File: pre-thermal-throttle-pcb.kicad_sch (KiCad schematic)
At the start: 70 parts, among them IC1 LMR51420XFDDCR, IC2 ADR02BRZ-REEL7, IC3 ADR02BRZ-REEL7, IC4 ADR02BRZ-REEL7, IC5 ADR02BRZ-REEL7, J1 RJHSE-5381-ND, J2 STEERING, J3 Motor Throttle Connector, J4 RJHSE-5381-ND, U1 SN65HVD230, U2 BMI088, U3 MAX3485CSA, U4 MCP3008, U5 ESP32-DevKitC

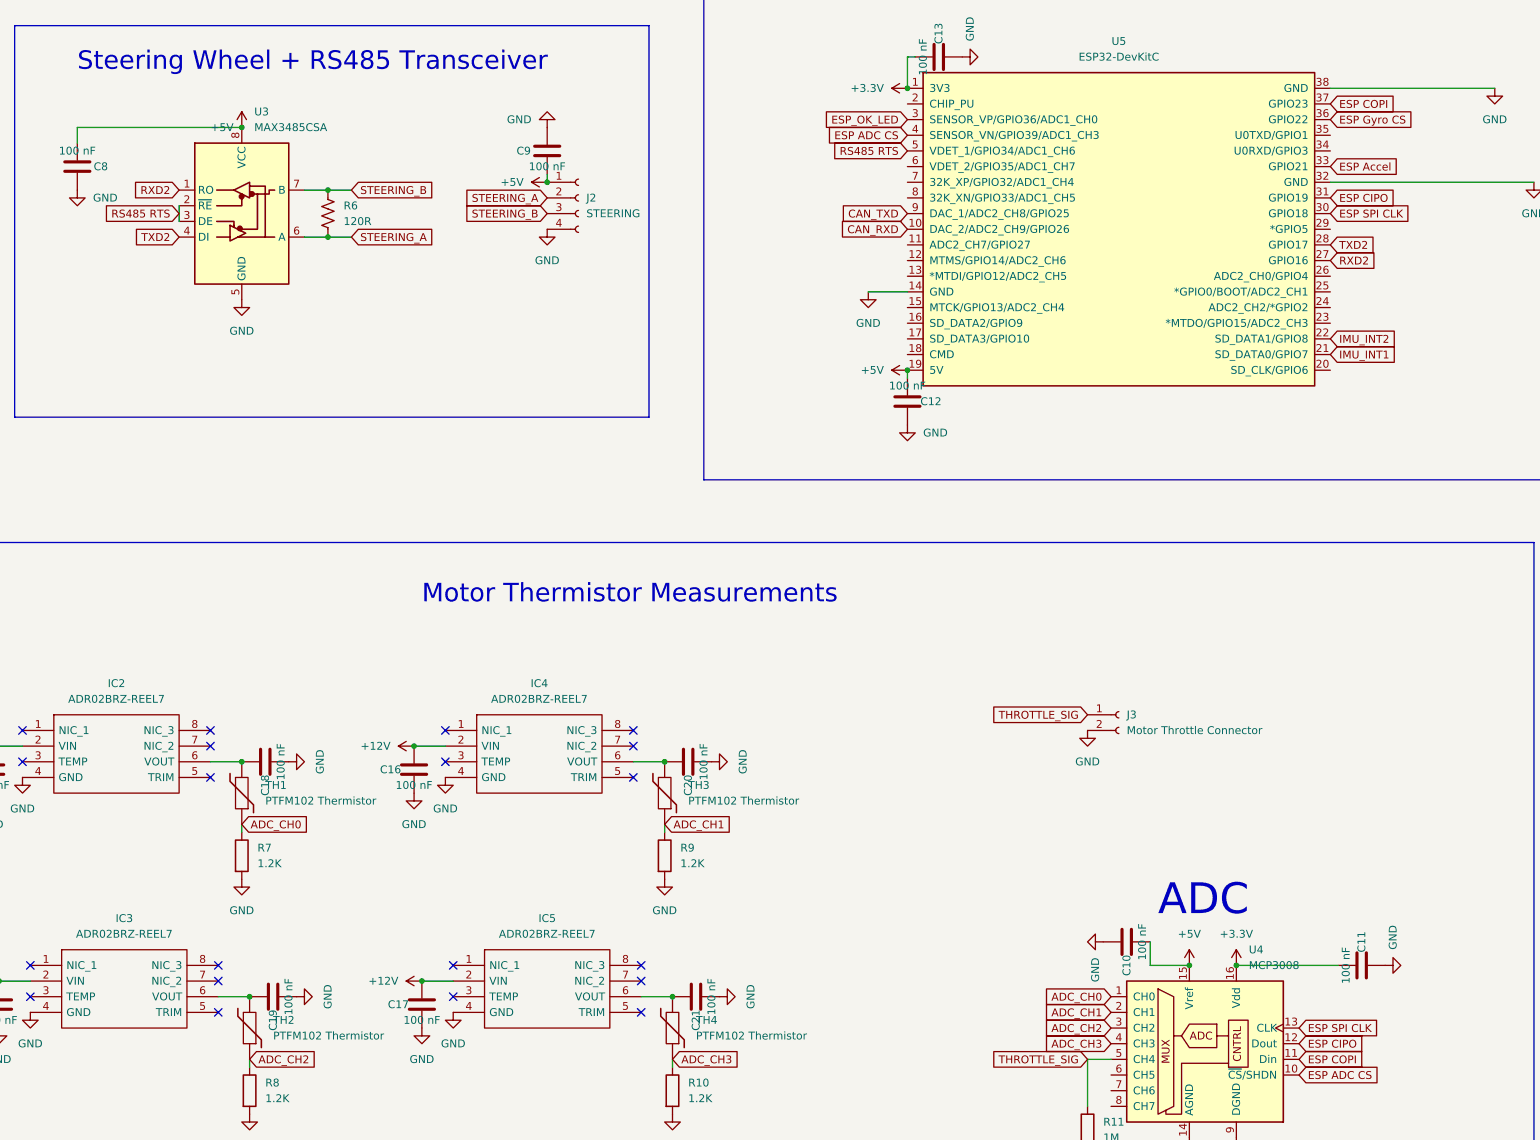
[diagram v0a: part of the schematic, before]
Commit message: Hopefully finished?
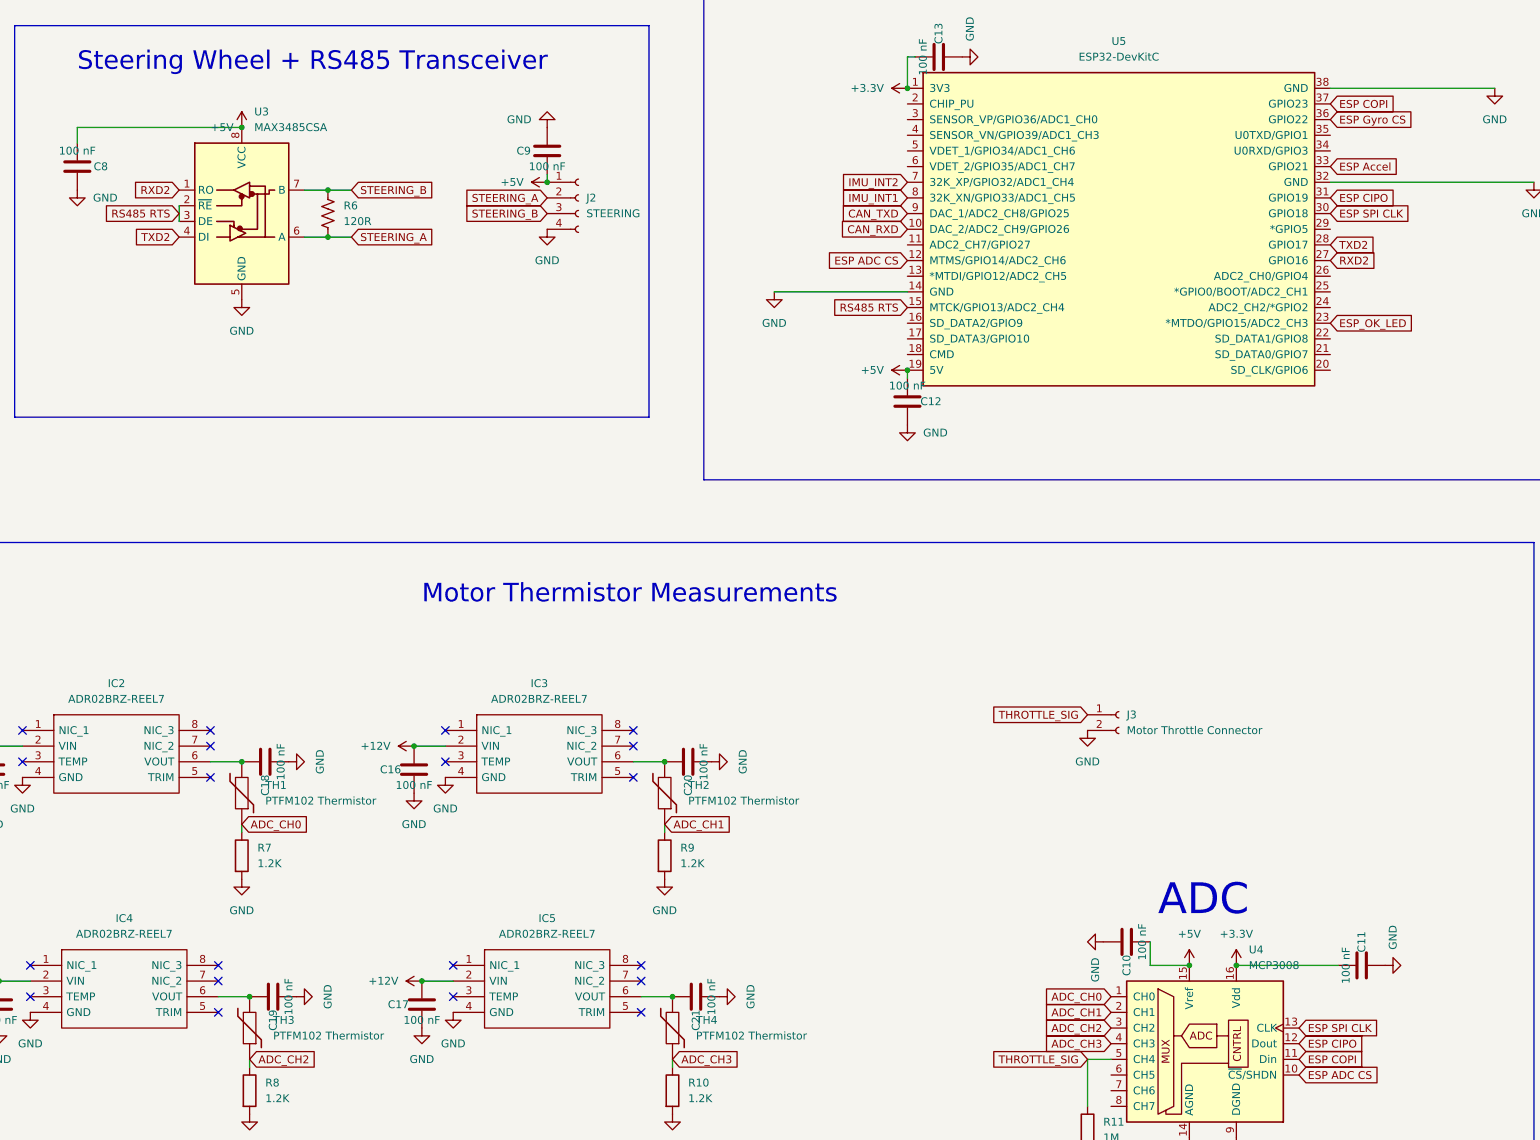
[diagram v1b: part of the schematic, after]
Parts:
- renumbered IC4 to IC3, IC3 to IC4, TH3 to TH2, TH2 to TH3
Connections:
- net ESP ADC CS: now also U5.12 (MTMS/GPIO14/ADC2_CH6); no longer U5.4 (SENSOR_VN/GPIO39/ADC1_CH3)
- net ESP_OK_LED: now also U5.23 (*MTDO/GPIO15/ADC2_CH3); no longer U5.3 (SENSOR_VP/GPIO36/ADC1_CH0)
- net IMU_INT1: now also U5.8 (32K_XN/GPIO33/ADC1_CH5); no longer U5.21 (SD_DATA0/GPIO7)
- net IMU_INT2: now also U5.7 (32K_XP/GPIO32/ADC1_CH4); no longer U5.22 (SD_DATA1/GPIO8)
- net RS485 RTS: now also U5.15 (MTCK/GPIO13/ADC2_CH4); no longer U5.5 (VDET_1/GPIO34/ADC1_CH6)
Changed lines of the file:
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@@
     (stroke (width 0) (type default) (color 0 0 0 0))
   )
-  (wire (pts (xy 302.26 233.68) (xy 308.61 233.68))
+  (wire (pts (xy 287.02 233.68) (xy 308.61 233.68))
     (stroke (width 0) (type default) (color 0 0 0 0))
   )
@@
     )
   )
+  (global_label "IMU_INT1" (shape input) (at 308.61 218.44 180) (fields_autoplaced)
+    (effects (font (size 1.27 1.27)) (justify right))
+    (property "Intersheet References" "${INTERSHEET_REFS}" (id 0) (at 297.7302 218.5194 0)
+      (effects (font (size 1.27 1.27)) (justify right) hide)
+    )
+  )
   (global_label "ESP SPI CLK" (shape input) (at 256.54 139.7 180) (fields_autoplaced)
     (effects (font (size 1.27 1.27)) (justify right))
@@
     )
   )
-  (global_label "IMU_INT2" (shape input) (at 377.19 241.3 0) (fields_autoplaced)
-    (effects (font (size 1.27 1.27)) (justify left))
-    (property "Intersheet References" "${INTERSHEET_REFS}" (id 0) (at 388.0698 241.2206 0)
-      (effects (font (size 1.27 1.27)) (justify left) hide)
-    )
-  )
   (global_label "STEERING_A" (shape input) (at 250.19 218.44 180) (fields_autoplaced)
     (effects (font (size 1.27 1.27)) (justify right))
@@
     )
   )
+  (global_label "RS485 RTS" (shape input) (at 308.61 236.22 180) (fields_autoplaced)
+    (effects (font (size 1.27 1.27)) (justify right))
+    (property "Intersheet References" "${INTERSHEET_REFS}" (id 0) (at 295.674 236.1406 0)
+      (effects (font (size 1.27 1.27)) (justify right) hide)
+    )
+  )
   (global_label "CAR_CANL" (shape input) (at 201.93 148.59 0) (fields_autoplaced)
     (effects (font (size 1.27 1.27)) (justify left))
@@
     )
   )
-  (global_label "IMU_INT1" (shape input) (at 377.19 243.84 0) (fields_autoplaced)
-    (effects (font (size 1.27 1.27)) (justify left))
-    (property "Intersheet References" "${INTERSHEET_REFS}" (id 0) (at 388.0698 243.7606 0)
-      (effects (font (size 1.27 1.27)) (justify left) hide)
-    )
-  )
   (global_label "CAN_TXD" (shape input) (at 167.64 143.51 180) (fields_autoplaced)
     (effects (font (size 1.27 1.27)) (justify right))
@@
     )
   )
+  (global_label "ESP_OK_LED" (shape input) (at 377.19 238.76 0) (fields_autoplaced)
+    (effects (font (size 1.27 1.27)) (justify left))
+    (property "Intersheet References" "${INTERSHEET_REFS}" (id 0) (at 391.2145 238.8394 0)
+      (effects (font (size 1.27 1.27)) (justify left) hide)
+    )
+  )
   (global_label "TXD2" (shape input) (at 190.5 224.79 180) (fields_autoplaced)
     (effects (font (size 1.27 1.27)) (justify right))
@@
     )
   )
-  (global_label "ESP Accel " (shape input) (at 256.54 132.08 180) (fields_autoplaced)
+  (global_label "IMU_INT2" (shape input) (at 308.61 215.9 180) (fields_autoplaced)
     (effects (font (size 1.27 1.27)) (justify right))
-    (property "Intersheet References" "${INTERSHEET_REFS}" (id 0) (at 243.5436 132.0006 0)
+    (property "Intersheet References" "${INTERSHEET_REFS}" (id 0) (at 297.7302 215.9794 0)
       (effects (font (size 1.27 1.27)) (justify right) hide)
     )
   )
-  (global_label "ADC_CH0" (shape input) (at 341.63 347.98 180) (fields_autoplaced)
+  (global_label "ESP Accel " (shape input) (at 256.54 132.08 180) (fields_autoplaced)
     (effects (font (size 1.27 1.27)) (justify right))
-    (property "Intersheet References" "${INTERSHEET_REFS}" (id 0) (at 330.8107 348.0594 0)
+    (property "Intersheet References" "${INTERSHEET_REFS}" (id 0) (at 243.5436 132.0006 0)
       (effects (font (size 1.27 1.27)) (justify right) hide)
     )
   )
-  (global_label "ESP ADC CS" (shape input) (at 308.61 208.28 180) (fields_autoplaced)
+  (global_label "ADC_CH0" (shape input) (at 341.63 347.98 180) (fields_autoplaced)
     (effects (font (size 1.27 1.27)) (justify right))
-    (property "Intersheet References" "${INTERSHEET_REFS}" (id 0) (at 294.525 208.3594 0)
+    (property "Intersheet References" "${INTERSHEET_REFS}" (id 0) (at 330.8107 348.0594 0)
       (effects (font (size 1.27 1.27)) (justify right) hide)
     )
@@
     )
   )
+  (global_label "ESP ADC CS" (shape input) (at 308.61 228.6 180) (fields_autoplaced)
+    (effects (font (size 1.27 1.27)) (justify right))
+    (property "Intersheet References" "${INTERSHEET_REFS}" (id 0) (at 294.525 228.6794 0)
+      (effects (font (size 1.27 1.27)) (justify right) hide)
+    )
+  )
   (global_label "ESP ADC CS" (shape input) (at 372.11 360.68 0) (fields_autoplaced)
     (effects (font (size 1.27 1.27)) (justify left))
@@
     )
   )
-  (global_label "RS485 RTS" (shape input) (at 308.61 210.82 180) (fields_autoplaced)
-    (effects (font (size 1.27 1.27)) (justify right))
-    (property "Intersheet References" "${INTERSHEET_REFS}" (id 0) (at 295.674 210.7406 0)
-      (effects (font (size 1.27 1.27)) (justify right) hide)
-    )
-  )
-  (global_label "ESP_OK_LED" (shape input) (at 308.61 205.74 180) (fields_autoplaced)
-    (effects (font (size 1.27 1.27)) (justify right))
-    (property "Intersheet References" "${INTERSHEET_REFS}" (id 0) (at 294.5855 205.6606 0)
-      (effects (font (size 1.27 1.27)) (justify right) hide)
-    )
-  )
   (global_label "ADC_CH1" (shape input) (at 269.24 320.04 0) (fields_autoplaced)
     (effects (font (size 1.27 1.27)) (justify left))
@@
   (symbol (lib_id "Device:Thermistor") (at 269.24 314.96 180) (unit 1)
     (in_bom yes) (on_board yes) (fields_autoplaced)
-    (property "Reference" "TH3" (id 0) (at 273.05 313.6899 0)
+    (property "Reference" "TH2" (id 0) (at 273.05 313.6899 0)
       (effects (font (size 1.27 1.27)) (justify right))
     )
@@
   (symbol (lib_id "Device:Thermistor") (at 201.93 353.06 180) (unit 1)
     (in_bom yes) (on_board yes) (fields_autoplaced)
-    (property "Reference" "TH2" (id 0) (at 205.74 351.7899 0)
+    (property "Reference" "TH3" (id 0) (at 205.74 351.7899 0)
       (effects (font (size 1.27 1.27)) (justify right))
     )
@@
     (pin "8")
   )
-  (symbol (lib_name "GND_4") (lib_id "power:GND") (at 302.26 233.68 0) (unit 1)
+  (symbol (lib_name "GND_4") (lib_id "power:GND") (at 287.02 233.68 0) (unit 1)
     (in_bom yes) (on_board yes) (fields_autoplaced)
-    (property "Reference" "#PWR055" (id 0) (at 302.26 240.03 0)
+    (property "Reference" "#PWR055" (id 0) (at 287.02 240.03 0)
       (effects (font (size 1.27 1.27)) hide)
     )
-    (property "Value" "GND" (id 1) (at 302.26 238.76 0))
-    (property "Footprint" "" (id 2) (at 302.26 233.68 0)
+    (property "Value" "GND" (id 1) (at 287.02 238.76 0))
+    (property "Footprint" "" (id 2) (at 287.02 233.68 0)
       (effects (font (size 1.27 1.27)) hide)
     )
-    (property "Datasheet" "" (id 3) (at 302.26 233.68 0)
+    (property "Datasheet" "" (id 3) (at 287.02 233.68 0)
       (effects (font (size 1.27 1.27)) hide)
     )
@@
   (symbol (lib_id "ADR02BRZ-REEL7:ADR02BRZ-REEL7") (at 166.37 342.9 0) (unit 1)
     (in_bom yes) (on_board yes) (fields_autoplaced)
-    (property "Reference" "IC3" (id 0) (at 181.61 335.28 0))
+    (property "Reference" "IC4" (id 0) (at 181.61 335.28 0))
     (property "Value" "ADR02BRZ-REEL7" (id 1) (at 181.61 337.82 0))
     (property "Footprint" "ADR02BRZ:SOIC127P600X175-8N" (id 2) (at 193.04 340.36 0)
@@
   (symbol (lib_id "ADR02BRZ-REEL7:ADR02BRZ-REEL7") (at 233.68 304.8 0) (unit 1)
     (in_bom yes) (on_board yes) (fields_autoplaced)
-    (property "Reference" "IC4" (id 0) (at 248.92 297.18 0))
+    (property "Reference" "IC3" (id 0) (at 248.92 297.18 0))
     (property "Value" "ADR02BRZ-REEL7" (id 1) (at 248.92 299.72 0))
     (property "Footprint" "ADR02BRZ:SOIC127P600X175-8N" (id 2) (at 260.35 302.26 0)
@@
       (reference "IC2") (unit 1) (value "ADR02BRZ-REEL7") (footprint "ADR02BRZ:SOIC127P600X175-8N")
     )
-    (path "/f03ea826-c55d-4d80-877e-6e35963a04f1"
+    (path "/f96b582d-5516-46fb-ba76-04ad2bfa00a2"
       (reference "IC3") (unit 1) (value "ADR02BRZ-REEL7") (footprint "ADR02BRZ:SOIC127P600X175-8N")
     )
-    (path "/f96b582d-5516-46fb-ba76-04ad2bfa00a2"
+    (path "/f03ea826-c55d-4d80-877e-6e35963a04f1"
       (reference "IC4") (unit 1) (value "ADR02BRZ-REEL7") (footprint "ADR02BRZ:SOIC127P600X175-8N")
     )
@@
       (reference "TH1") (unit 1) (value "PTFM102 Thermistor") (footprint "Connector_JST:JST_XH_B2B-XH-A_1x02_P2.50mm_Vertical")
     )
-    (path "/7475f588-3355-4f14-b57e-88cef5629661"
+    (path "/4ec6308e-6715-4c65-8fe8-dd6e13246823"
       (reference "TH2") (unit 1) (value "PTFM102 Thermistor") (footprint "Connector_JST:JST_XH_B2B-XH-A_1x02_P2.50mm_Vertical")
     )
-    (path "/4ec6308e-6715-4c65-8fe8-dd6e13246823"
+    (path "/7475f588-3355-4f14-b57e-88cef5629661"
       (reference "TH3") (unit 1) (value "PTFM102 Thermistor") (footprint "Connector_JST:JST_XH_B2B-XH-A_1x02_P2.50mm_Vertical")
     )

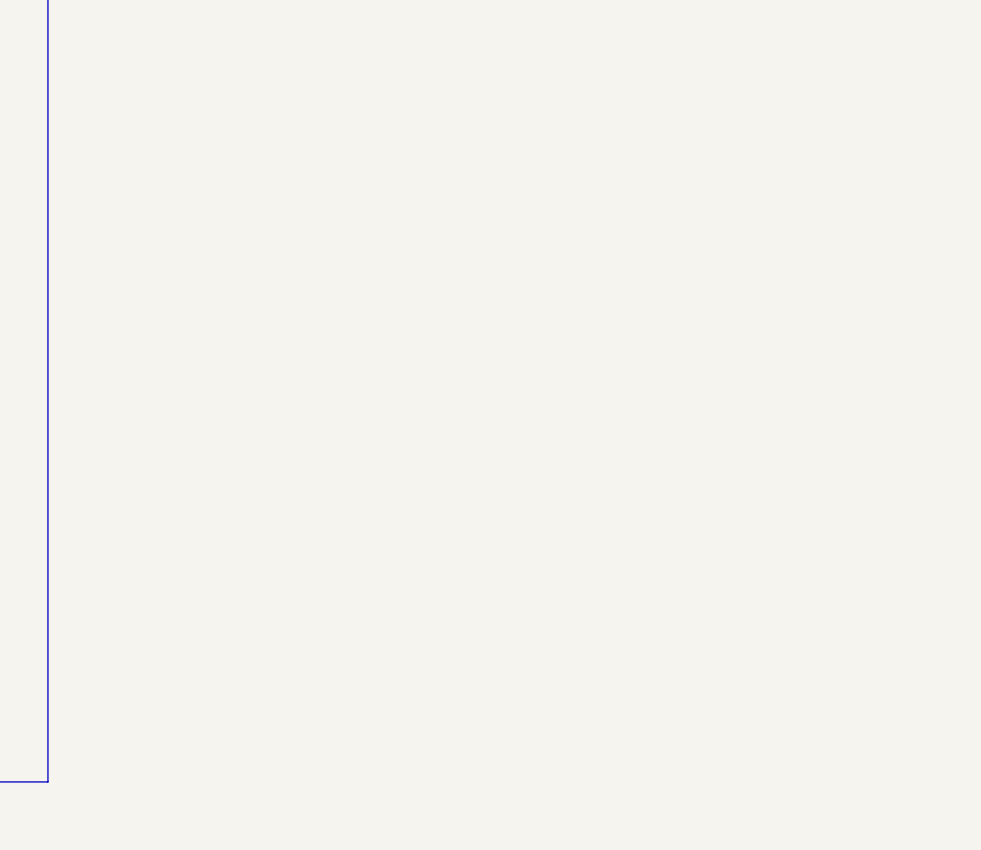
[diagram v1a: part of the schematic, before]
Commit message: Muh silkscreen
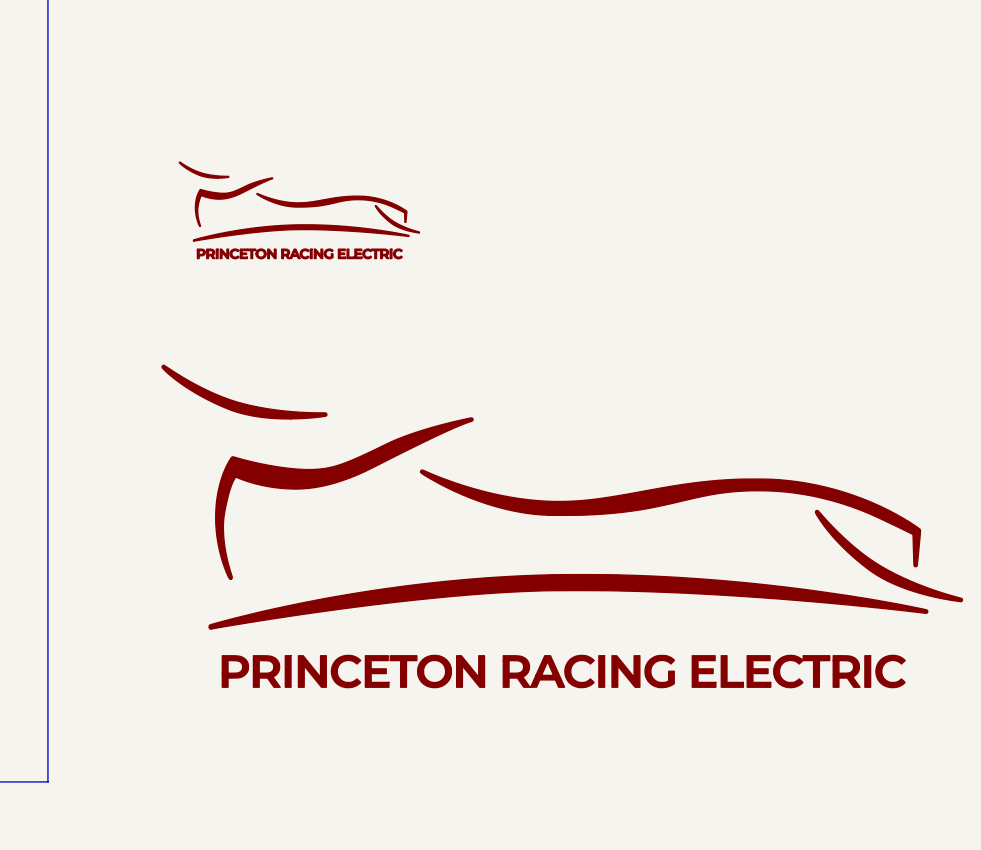
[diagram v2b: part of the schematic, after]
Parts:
- added G1: LOGO, pre_logo:pre_logo_medium, symbol pre_logo_medium:LOGO
- added G2: LOGO, pre_logo:pre_logo_big, symbol pre_logo_big:LOGO
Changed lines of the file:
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@@
     (pin "1")
+  )
+  (symbol (lib_id "pre_logo_medium:LOGO") (at 449.58 201.93 0) (unit 1)
+    (in_bom yes) (on_board yes) (fields_autoplaced)
+    (property "Reference" "G1" (id 0) (at 449.58 193.5643 0)
+      (effects (font (size 1.27 1.27)) hide)
+    )
+    (property "Value" "LOGO" (id 1) (at 449.58 210.2957 0)
+      (effects (font (size 1.27 1.27)) hide)
+    )
+    (property "Footprint" "pre_logo:pre_logo_medium" (id 2) (at 449.58 201.93 0)
+      (effects (font (size 1.27 1.27)) hide)
+    )
+    (property "Datasheet" "" (id 3) (at 449.58 201.93 0)
+      (effects (font (size 1.27 1.27)) hide)
+    )
   )
   (symbol (lib_id "power:GND") (at 54.61 336.55 0) (unit 1)
@@
     (pin "2")
   )
+  (symbol (lib_id "pre_logo_big:LOGO") (at 478.79 240.03 0) (unit 1)
+    (in_bom yes) (on_board yes) (fields_autoplaced)
+    (property "Reference" "G2" (id 0) (at 478.79 210.6414 0)
+      (effects (font (size 1.27 1.27)) hide)
+    )
+    (property "Value" "LOGO" (id 1) (at 478.79 269.4186 0)
+      (effects (font (size 1.27 1.27)) hide)
+    )
+    (property "Footprint" "pre_logo:pre_logo_big" (id 2) (at 478.79 240.03 0)
+      (effects (font (size 1.27 1.27)) hide)
+    )
+    (property "Datasheet" "" (id 3) (at 478.79 240.03 0)
+      (effects (font (size 1.27 1.27)) hide)
+    )
+  )
   (symbol (lib_name "GND_2") (lib_id "power:GND") (at 200.66 234.95 0) (unit 1)
     (in_bom yes) (on_board yes) (fields_autoplaced)
@@
       (reference "CREGout1") (unit 1) (value "47uF") (footprint "Capacitor_SMD:C_0805_2012Metric")
     )
+    (path "/6fd919b7-1f24-43be-832a-764aaf94eea8"
+      (reference "G1") (unit 1) (value "LOGO") (footprint "pre_logo:pre_logo_medium")
+    )
+    (path "/95261407-4cf8-4722-9fff-9bee7548a6b8"
+      (reference "G2") (unit 1) (value "LOGO") (footprint "pre_logo:pre_logo_big")
+    )
     (path "/27742449-baf5-4df5-878c-9fc704c1da42"
